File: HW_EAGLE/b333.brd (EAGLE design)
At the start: 80 x 50.5 mm, 158 parts, among them Q1 2N4126, Q2 2N4126, X1 USB MICRO, X2 USB MICRO

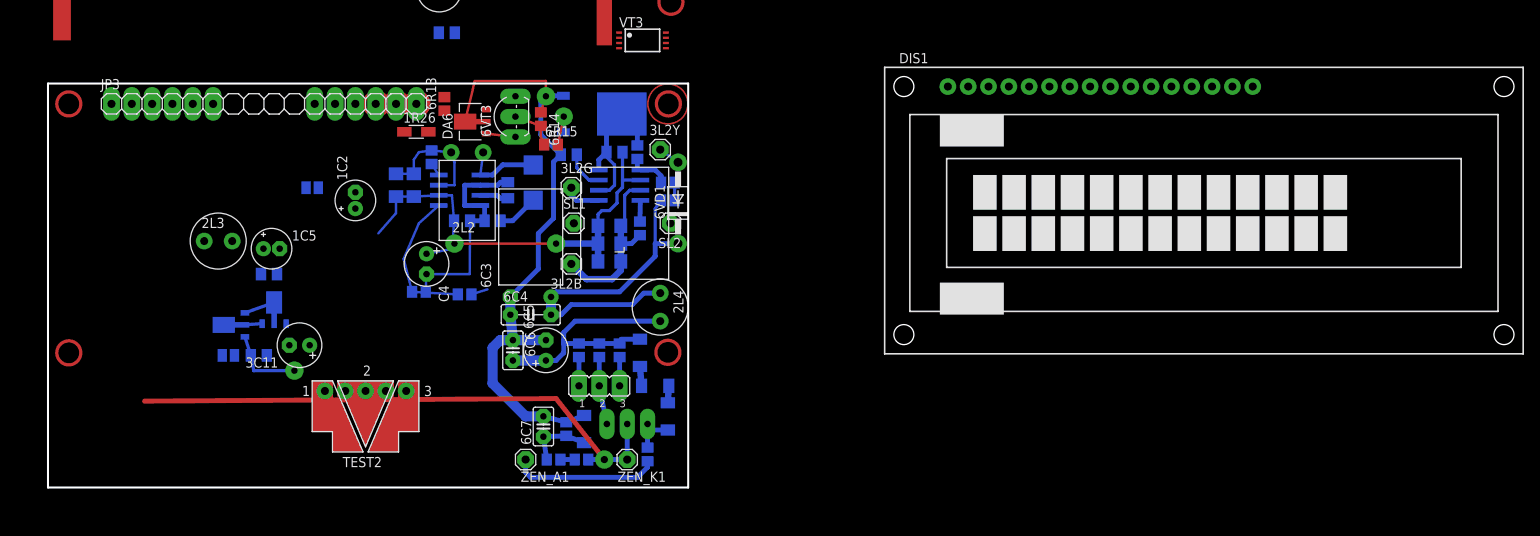
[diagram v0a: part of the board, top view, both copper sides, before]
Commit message: .
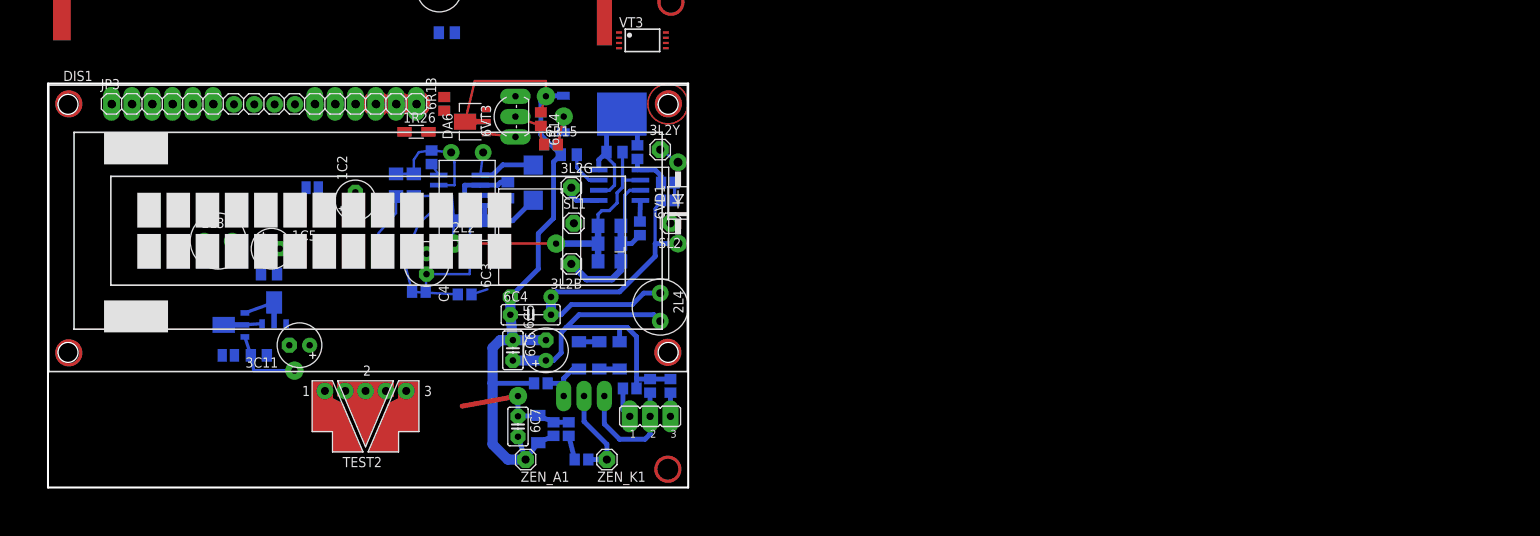
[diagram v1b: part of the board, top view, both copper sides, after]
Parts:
- removed D1: (no value), diode:SOD80C
- added Z1: 5v6, diode:SOD80C
- moved DIS1 104.5 mm to (191.8, 94.6)
- moved 6R9 16.0 mm to (213.4, 75.2), turned to 180 degrees
- moved 6VD4 13.5 mm to (218.1, 78.7)
- moved 6VD3 7.96 mm to (220.7, 78.7), turned to 270 degrees
- moved 6R6 7.94 mm to (224.5, 74.6), turned to 0 degrees
- moved 6R8 7.75 mm to (229.6, 74.9)
- moved 6R7 7.75 mm to (227.0, 74.9)
- moved 5MA 7.41 mm to (227.0, 71.1)
- moved VT6 6.43 mm to (218.8, 73.7), turned to 0 degrees
- moved 6R11 4.26 mm to (216.9, 69.5), turned to 270 degrees
- moved 6C7 3.18 mm to (210.5, 69.8), turned to 270 degrees
- moved 6VD2 2.56 mm to (223.2, 78.7)
- moved ZEN_K1 2.54 mm to (221.6, 65.7)
- moved 6R12 1.59 mm to (214.9, 69.5), turned to 90 degrees
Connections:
- net GND: now also Z1.A; no longer D1.A
- net PC3: now also DD1.26, Z1.C; no longer D1.C
- net ZENER: no longer DD1.26
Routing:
- net ZENER: track 70.5 -> 11.4 mm, vias 1 -> 0
- net +90.5V: track 31.8 -> 44.4 mm
- net PC3: track 8.13 -> 16.2 mm, vias 0 -> 1
- net 1MA: track 8.45 -> 15.4 mm
- net GND: track 299.1 -> 292.8 mm
- net N$24: track 1.79 -> 3.05 mm
- net N$55: track 3.59 -> 2.96 mm
